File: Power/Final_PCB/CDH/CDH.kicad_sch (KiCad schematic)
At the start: 17 parts, among them IC1 TEENSY_4.1, J1 Left_Header, J2 Right_Header, J3 Transceiver header, U3 DPS310XTSA1, U4 HTS221

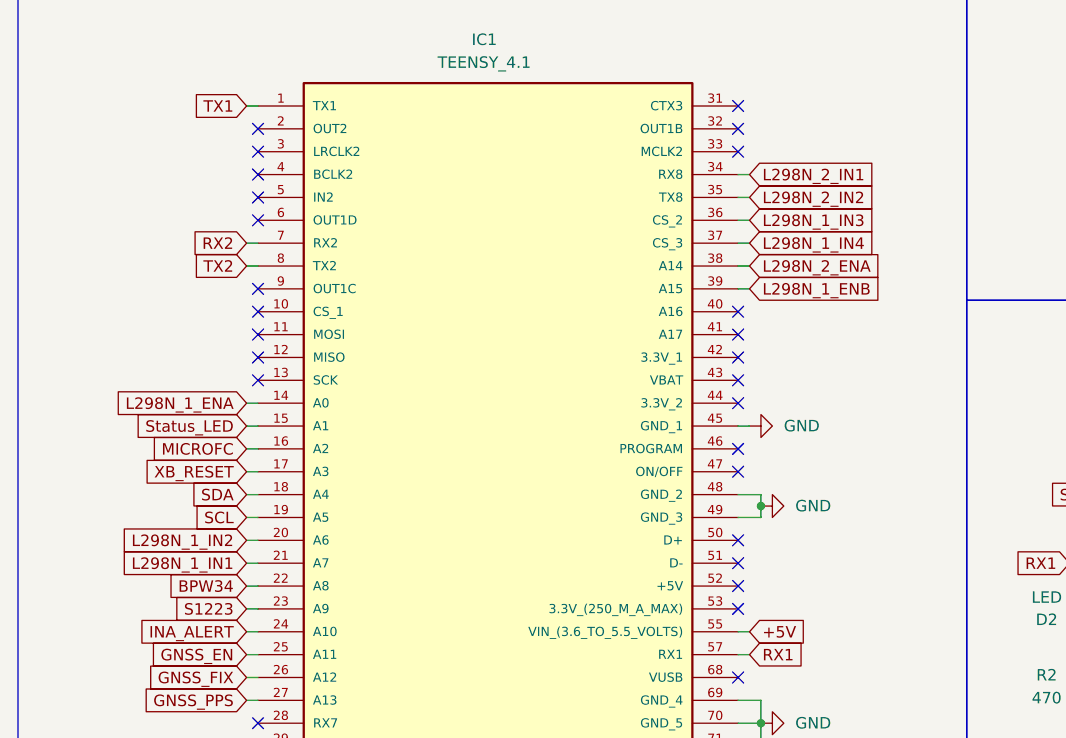
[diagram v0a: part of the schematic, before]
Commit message: Completed CDH Board
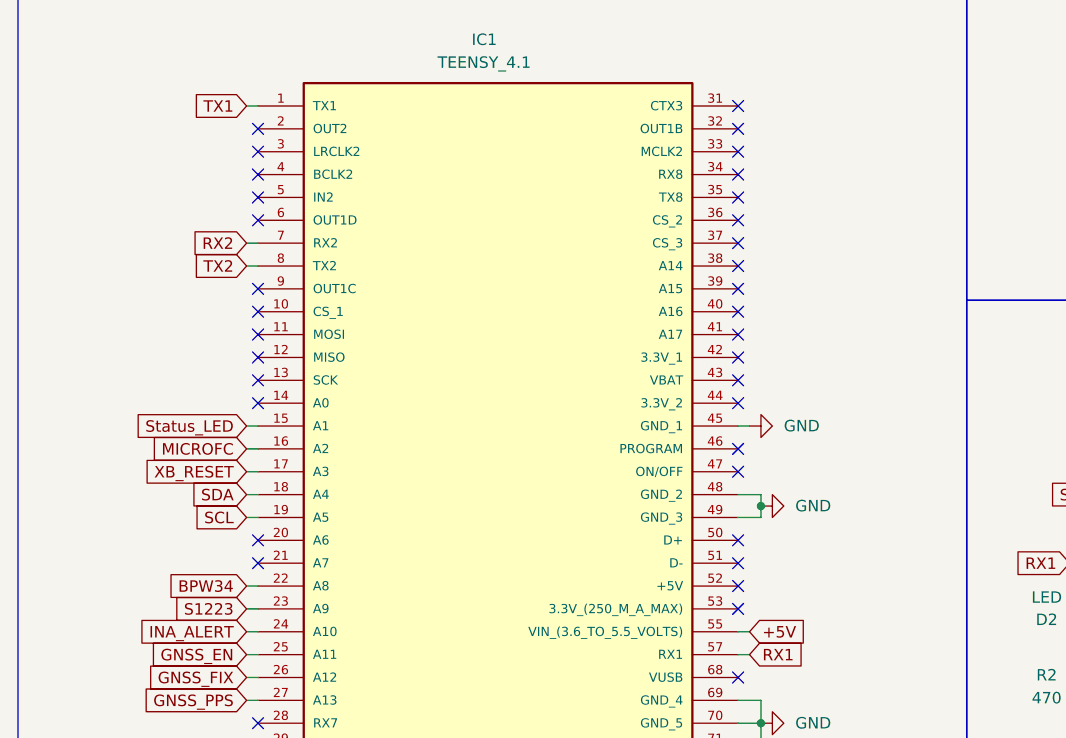
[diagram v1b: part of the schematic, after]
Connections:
- net L298N_1_ENA: no longer names the net of IC1.14 (A0)
- net L298N_1_ENB: no longer names the net of IC1.39 (A15)
- net L298N_1_IN1: no longer names the net of IC1.21 (A7)
- net L298N_1_IN2: no longer names the net of IC1.20 (A6)
- net L298N_1_IN3: no longer names the net of IC1.36 (CS_2)
- net L298N_1_IN4: no longer names the net of IC1.37 (CS_3)
- net L298N_2_ENA: no longer names the net of IC1.38 (A14)
- net L298N_2_IN1: no longer names the net of IC1.34 (RX8)
- net L298N_2_IN2: no longer names the net of IC1.35 (TX8)
- no-connect marks 50 -> 59

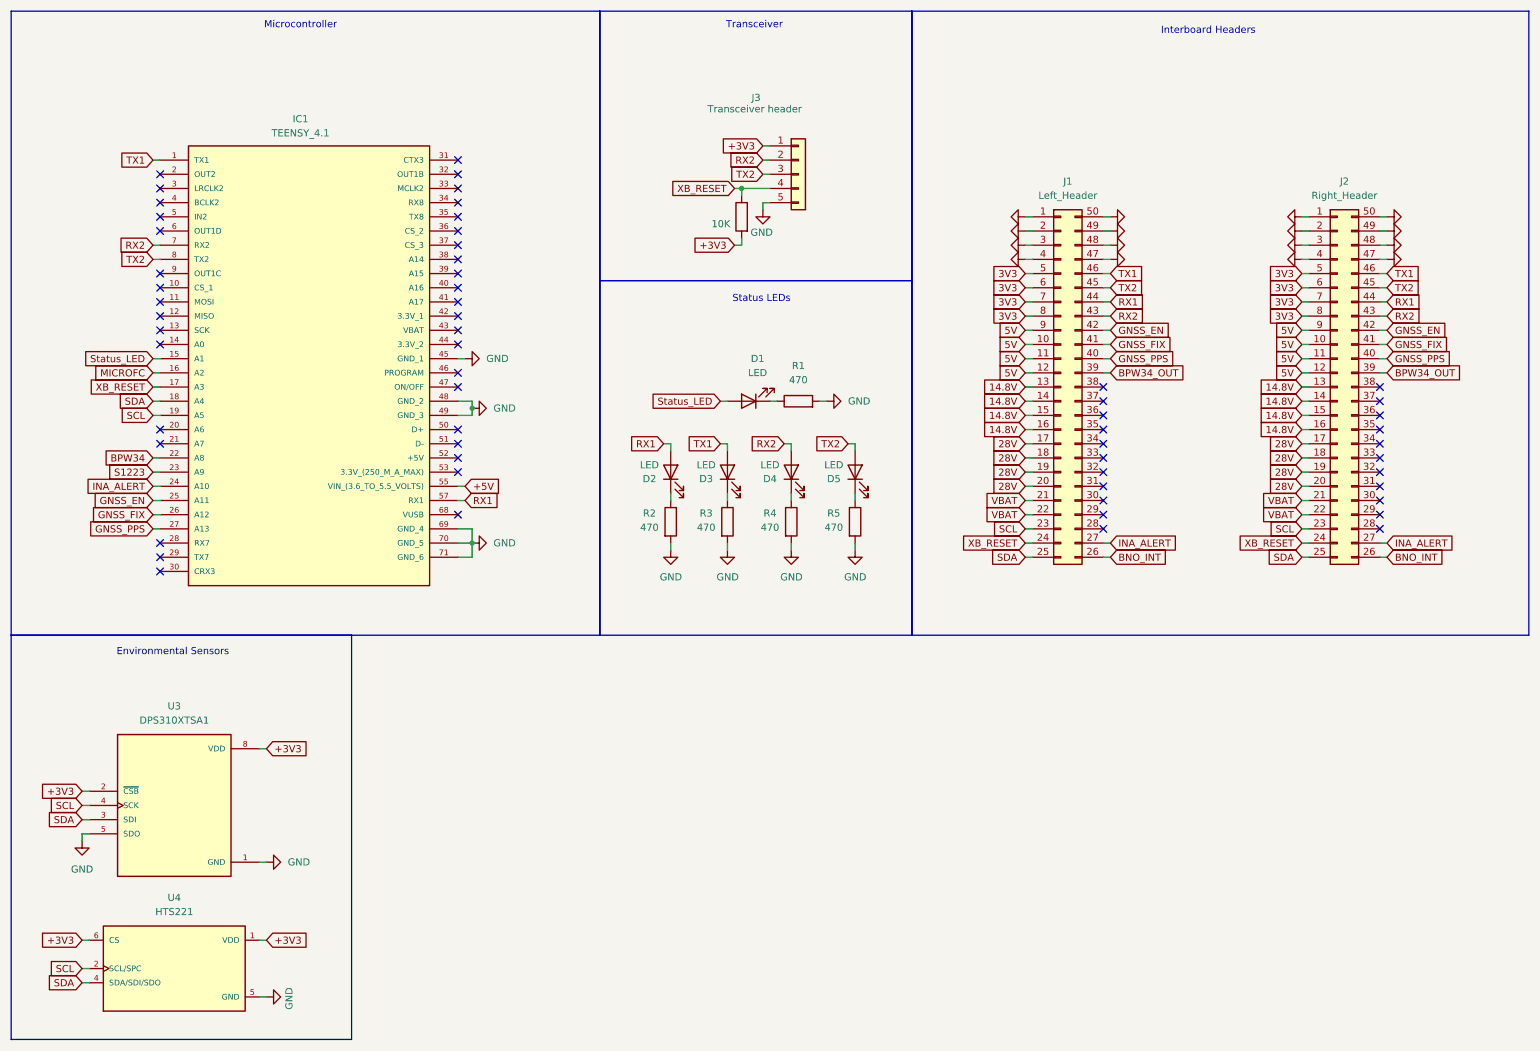
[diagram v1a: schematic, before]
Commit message: Finalising Sensors Schematic
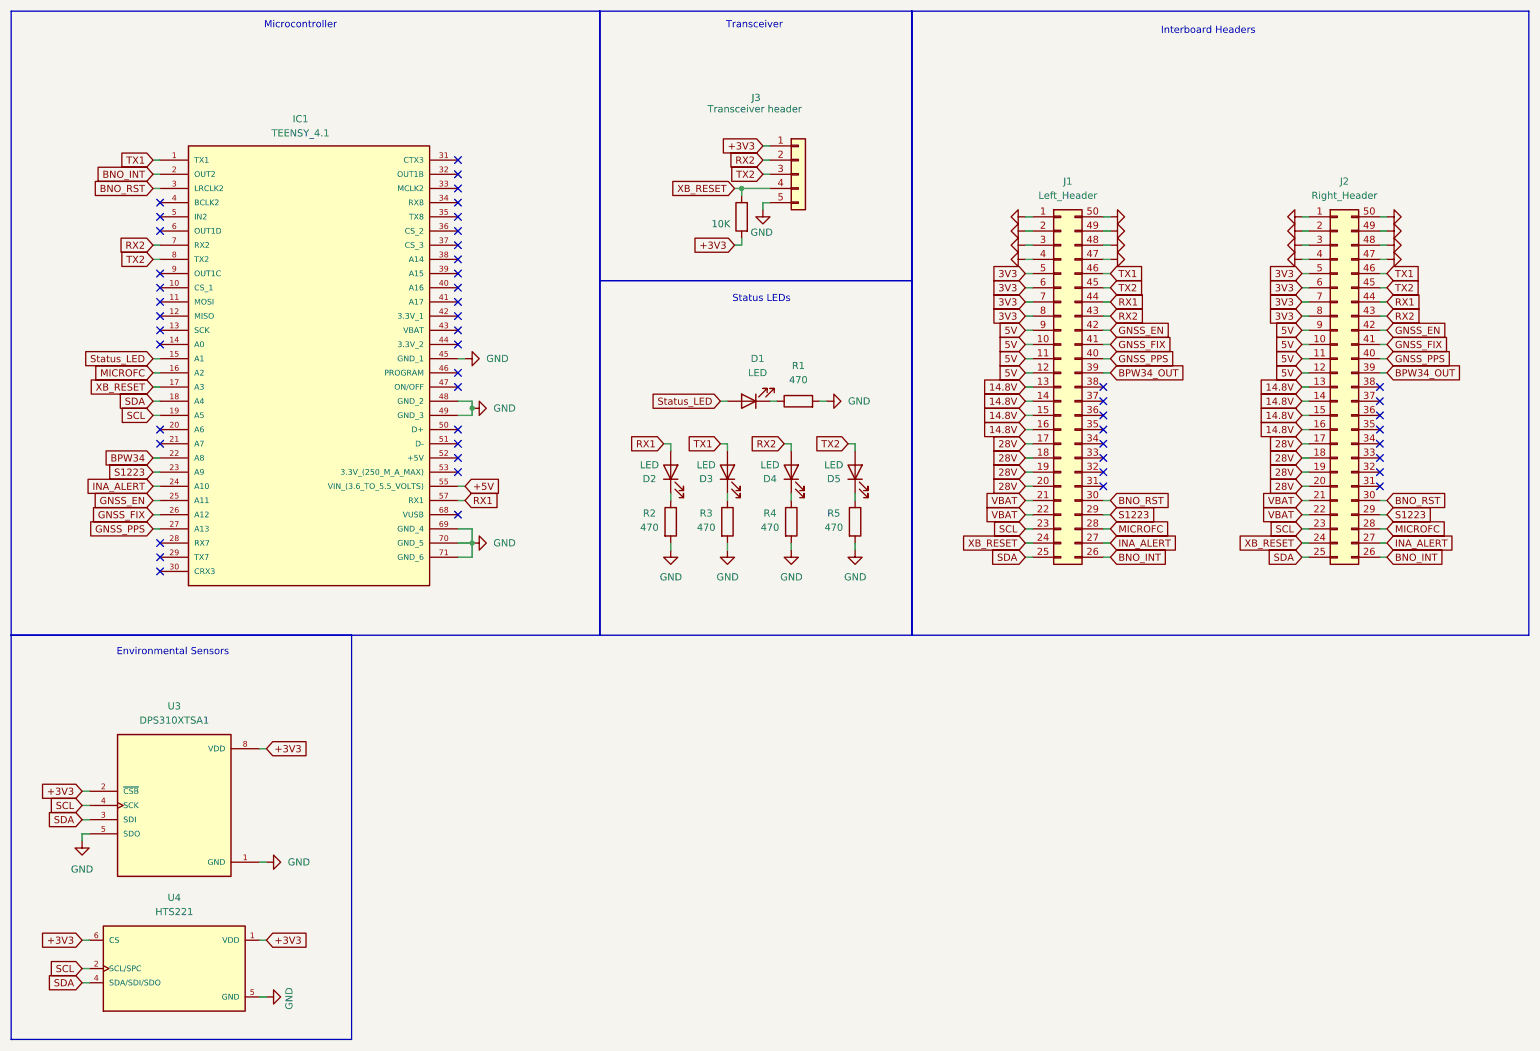
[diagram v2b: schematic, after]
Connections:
- net BNO_INT: now also IC1.2 (OUT2)
- net MICROFC: now also J1.28 (Pin_28), J2.28 (Pin_28)
- net S1223: now also J1.29 (Pin_29), J2.29 (Pin_29)
- net BNO_RST: now reaches J2.30 (Pin_30)
- net BNO_RST: now also IC1.3 (LRCLK2), J1.30 (Pin_30)
- no-connect marks 59 -> 51
